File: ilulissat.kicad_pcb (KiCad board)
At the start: 2 copper layers, 25.4 x 25.4 mm, 30 parts, among them SW1 SW_SPST, U1 EFR32MG21x, U2 HDC2080, Y1 32.768Khz, Y2 38.4Mhz

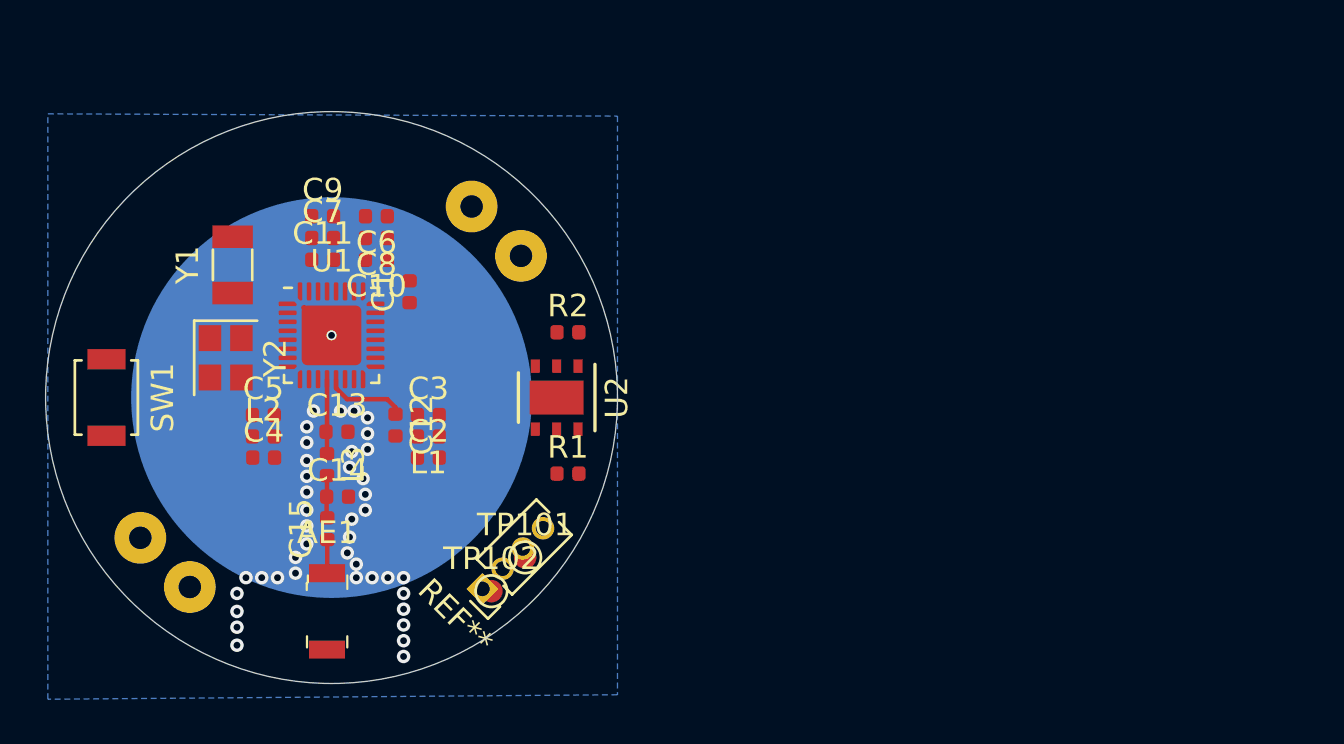
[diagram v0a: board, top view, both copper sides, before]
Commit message: arg
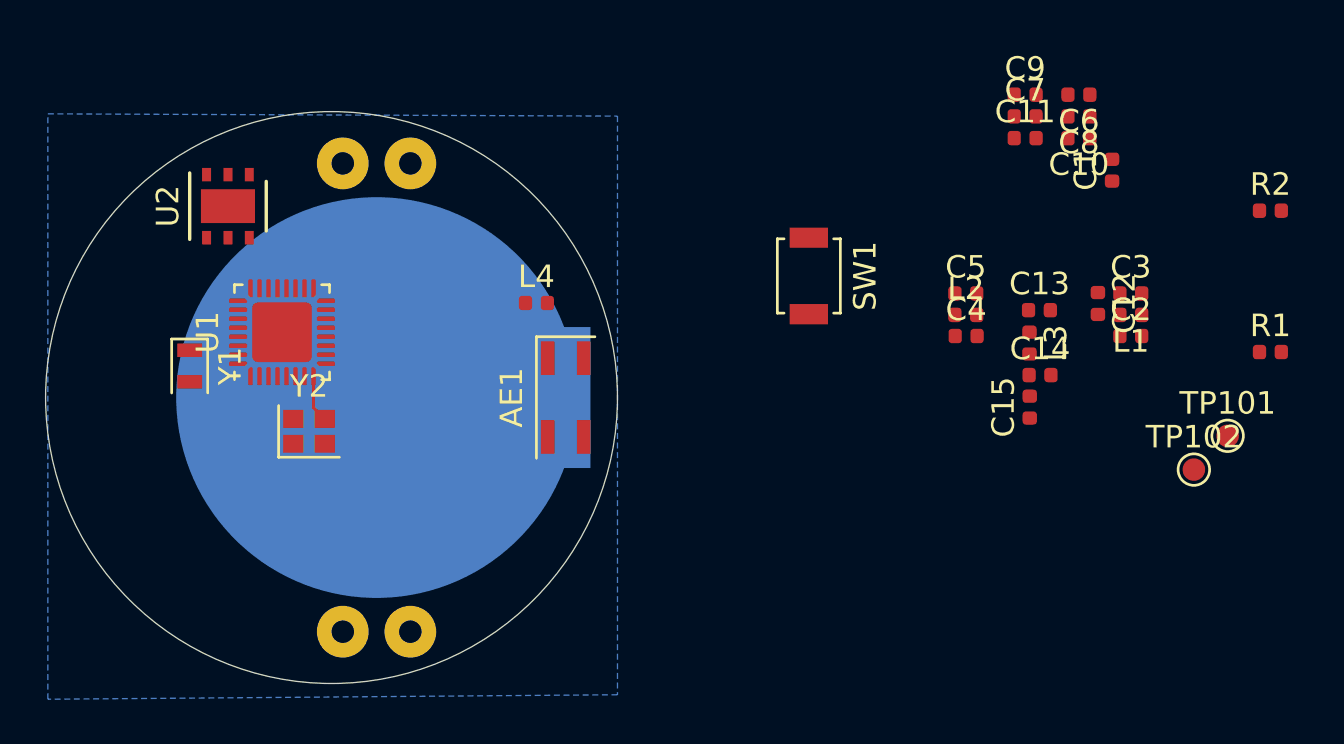
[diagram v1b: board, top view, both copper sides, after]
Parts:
- removed REF**: PinHeader_1x04_P1.27mm_Vertical, Connector_PinHeader_1.27mm:PinHeader_1x04_P1.27mm_Vertical
- added L4: 0R, Inductor_SMD:L_0402_1005Metric, F.Cu at (159.1, 95.8)
- AE1: footprint Antenna_Extra:2450AT18A100 -> Antenna_Extra:Antenna_Johanson_2450AT42E0100
- BT1: footprint batt:BAT-HLD-001-THM -> batt:BatteryHolder_Linx_BAT-HLD-001-THM
- Y1: footprint Crystal:Crystal_SMD_3215-2Pin_3.2x1.5mm -> Crystal:Crystal_SMD_2012-2Pin_2.0x1.2mm
- Y2: footprint Crystal:Crystal_SMD_2520-4Pin_2.5x2.0mm -> Crystal:Crystal_SMD_2016-4Pin_2.0x1.6mm
- moved C10 31.7 mm to (183.2, 88.5)
- moved C11 31.7 mm to (180.8, 88.5)
- moved C12 31.7 mm to (184.0, 95.8)
- moved C13 31.7 mm to (181.4, 96.1)
- moved C4 31.7 mm to (178.2, 97.3)
- moved C5 31.7 mm to (178.2, 95.4)
- moved C6 31.7 mm to (183.2, 86.5)
- moved C7 31.7 mm to (180.8, 87.5)
- moved C8 31.7 mm to (183.2, 87.5)
- moved C9 31.7 mm to (180.8, 86.5)
- moved L2 31.7 mm to (178.2, 96.3)
- moved L3 31.7 mm to (181.0, 97.6)
- moved TP101 31.7 mm to (189.8, 101.7)
- moved TP102 31.7 mm to (188.3, 103.2)
- moved C14 31.7 mm to (181.5, 99.0)
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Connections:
- net Net-(C2-Pad1) renamed /PAVDD
- net Net-(C4-Pad2) renamed /RFVDD
- net Net-(U1-Pad31) renamed /LFXTAL_I
- net Net-(U1-Pad32) renamed /LFXTAL_O
- net Net-(U1-Pad7) renamed /HFXTAL_I
- net Net-(U1-Pad8) renamed /HFXTAL_O
- AE1 pad 2: Net-(AE1-Pad2) -> GND
- C15 pad 1: Net-(AE1-Pad1) -> Net-(C15-Pad1)
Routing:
- net /ANT-: track 3.68 -> 0.00 mm
- net /ANT+: track 3.34 -> 0.00 mm
- net /HFXTAL_O: track 0.00 -> 2.11 mm
- net Net-(C14-Pad1): track 1.89 -> 0.00 mm
- net GND: track 1.73 -> 0.00 mm, vias 42 -> 0
- net Net-(AE1-Pad1): track 1.49 -> 0.00 mm

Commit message: Routing complete, needs cleanup
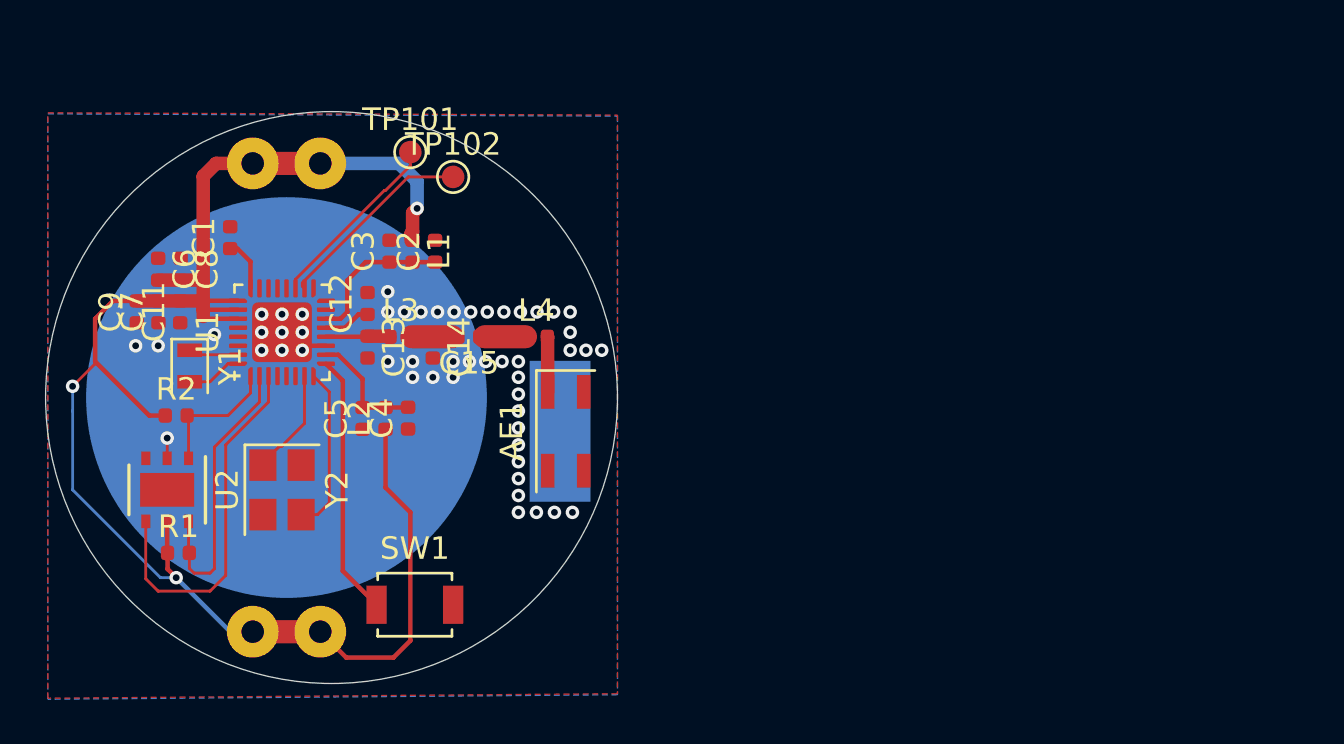
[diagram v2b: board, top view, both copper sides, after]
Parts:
- removed C10: 10uF, Capacitor_SMD:C_0402_1005Metric
- Y2: footprint Crystal:Crystal_SMD_2016-4Pin_2.0x1.6mm -> Crystal:Crystal_SMD_3225-4Pin_3.2x2.5mm
- moved R2 49.4 mm to (143.1, 100.8)
- moved R1 49.3 mm to (143.2, 106.9)
- moved C6 41.6 mm to (142.3, 94.3), turned to 270 degrees
- moved C9 40.6 mm to (141.3, 96.2), turned to 90 degrees
- moved C8 40.5 mm to (143.3, 94.3), turned to 270 degrees
- moved C7 39.5 mm to (142.3, 96.2), turned to 90 degrees
- moved C1 39.3 mm to (145.5, 92.9)
- moved TP101 38.4 mm to (153.5, 89.1)
- moved C11 38.3 mm to (143.3, 96.2), turned to 90 degrees
- moved TP102 35.4 mm to (155.4, 90.2)
- moved C3 33.0 mm to (152.6, 93.5), turned to 90 degrees
- moved C12 32.4 mm to (151.6, 95.8), turned to 90 degrees
- moved L1 32.0 mm to (153.6, 93.5), turned to 270 degrees
- moved C2 31.1 mm to (154.6, 93.5), turned to 90 degrees
- moved C13 29.9 mm to (151.6, 97.8), turned to 270 degrees
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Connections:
- U1 pad 1: Net-(U1-Pad1) -> /HDC_SDA
- U1 pad 2: Net-(U1-Pad2) -> /HDC_SCL
- U1 pad 21: /HDC_SCL -> Net-(U1-Pad21)
- U1 pad 22: /HDC_INT -> Net-(U1-Pad22)
- U1 pad 23: /HDC_SDA -> Net-(U1-Pad23)
- U1 pad 3: Net-(U1-Pad3) -> /HDC_INT
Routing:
- net VDD: track 0.00 -> 73.9 mm, vias 0 -> 3
- net /HDC_INT: track 0.00 -> 16.3 mm
- net /HDC_SCL: track 0.00 -> 12.8 mm
- net /~RESET~: track 0.00 -> 11.6 mm
- net /SWCLK: track 0.00 -> 8.93 mm
- net /SWDIO: track 0.00 -> 8.19 mm
- net /PAVDD: track 0.00 -> 6.64 mm
- net /HDC_SDA: track 0.00 -> 5.91 mm
- net /RFVDD: track 0.00 -> 5.31 mm
- net /HFXTAL_O: track 2.11 -> 7.38 mm
- net /HFXTAL_I: track 0.00 -> 4.77 mm
- net /ANT+: track 0.00 -> 2.87 mm
- net /LFXTAL_O: track 0.00 -> 2.48 mm
- net Net-(AE1-Pad1): track 0.00 -> 2.46 mm
- net Net-(C1-Pad1): track 0.00 -> 2.33 mm
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- added copper zone on F.Cu, net GND
